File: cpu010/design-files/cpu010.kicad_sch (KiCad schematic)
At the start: 12 parts

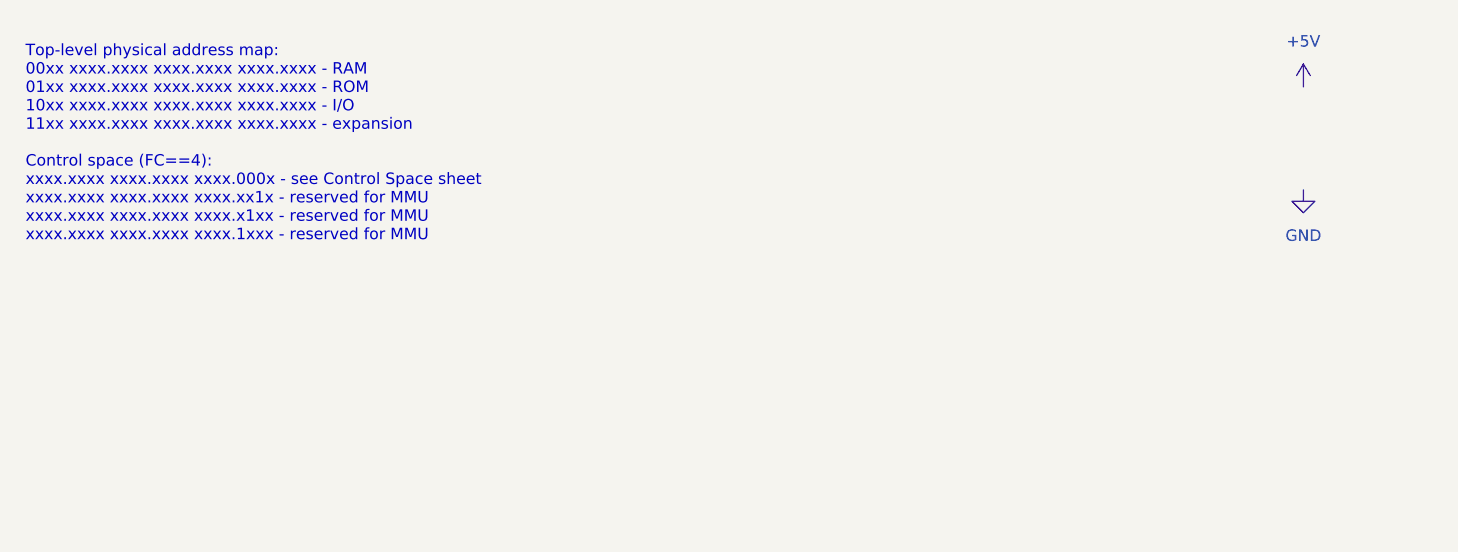
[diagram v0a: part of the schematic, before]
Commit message: More (NQ)VME tweaks.  Add JTAG chain.
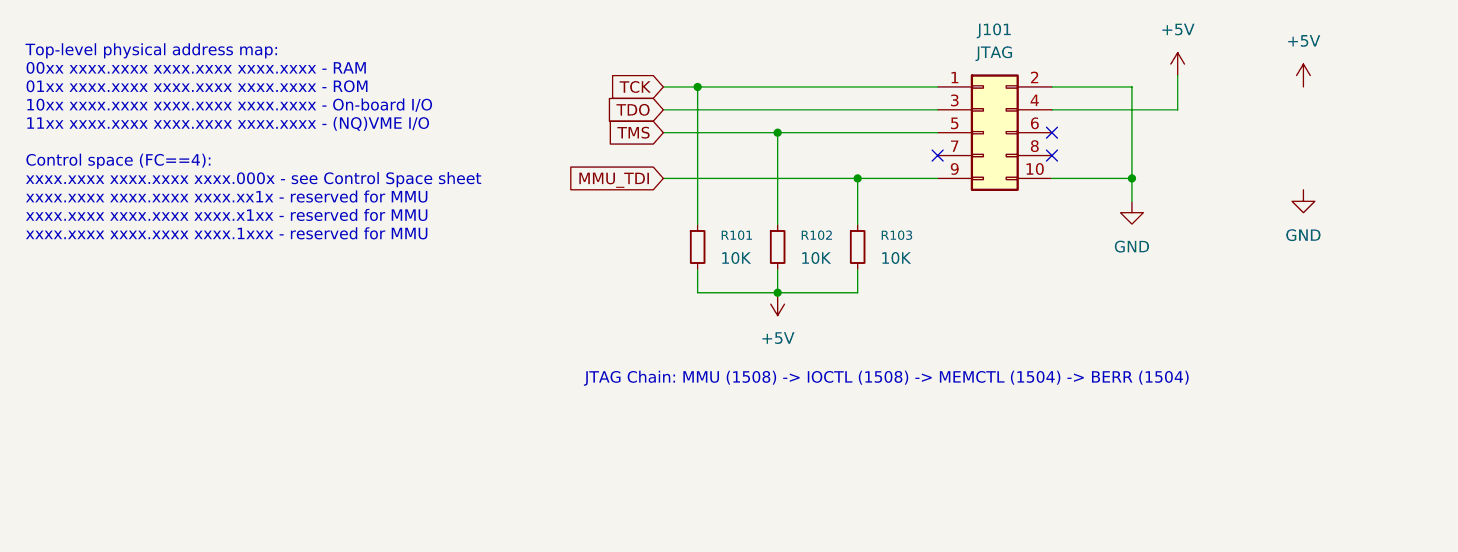
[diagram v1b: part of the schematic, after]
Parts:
- added J101: JTAG, Connector_PinHeader_2.54mm:PinHeader_2x05_P2.54mm_Vertical, symbol Connector_Generic:Conn_02x05_Odd_Even
- added R101, R102, R103: 10K, Resistor_SMD:R_0805_2012Metric_Pad1.20x1.40mm_HandSolder, symbol Device:R_Small
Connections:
- net +5V: now also J101.4 (Pin_4), R101.2, R102.2, R103.2
- net GND: now also J101.10 (Pin_10), J101.2 (Pin_2)
- new net MMU_TDI: J101.9 (Pin_9), R103.1
- new net TCK: J101.1 (Pin_1), R101.1
- new net TDO: J101.3 (Pin_3)
- new net TMS: J101.5 (Pin_5), R102.1
- no-connect marks 0 -> 3
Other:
- note added: "JTAG Chain: MMU (1508) -> IOCTL (1508) -> MEMCTL (1504) -> BERR (1504)"
- note added: "Top-level physical address map: 00xx xxxx.xxxx xxxx.xxxx xxxx.xxxx - RAM 01xx xxxx.xxxx xxxx.xxxx xxxx.xxxx - ROM 10xx xxxx.xxxx xxxx.xxxx xxxx.xxxx - On-board I/O 11xx xxxx.xxxx xxxx.xxxx xxxx.xxxx - (NQ)VME I/O Control space (FC==4): xxxx.xxxx xxxx.xxxx xxxx.000x - see Control Space sheet xxxx.xxxx xxxx.xxxx xxxx.xx1x - reserved for MMU xxxx.xxxx xxxx.xxxx xxxx.x1xx - reserved for MMU xxxx.xxxx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"
- note removed: "Top-level physical address map: 00xx xxxx.xxxx xxxx.xxxx xxxx.xxxx - RAM 01xx xxxx.xxxx xxxx.xxxx xxxx.xxxx - ROM 10xx xxxx.xxxx xxxx.xxxx xxxx.xxxx - I/O 11xx xxxx.xxxx xxxx.xxxx xxxx.xxxx - expansion Control space (FC==4): xxxx.xxxx xxxx.xxxx xxxx.000x - see Control Space sheet xxxx.xxxx xxxx.xxxx xxxx.xx1x - reserved for MMU xxxx.xxxx xxxx.xxxx xxxx.x1xx - reserved for MMU xxxx.xxxx xxxx.xxxx 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"

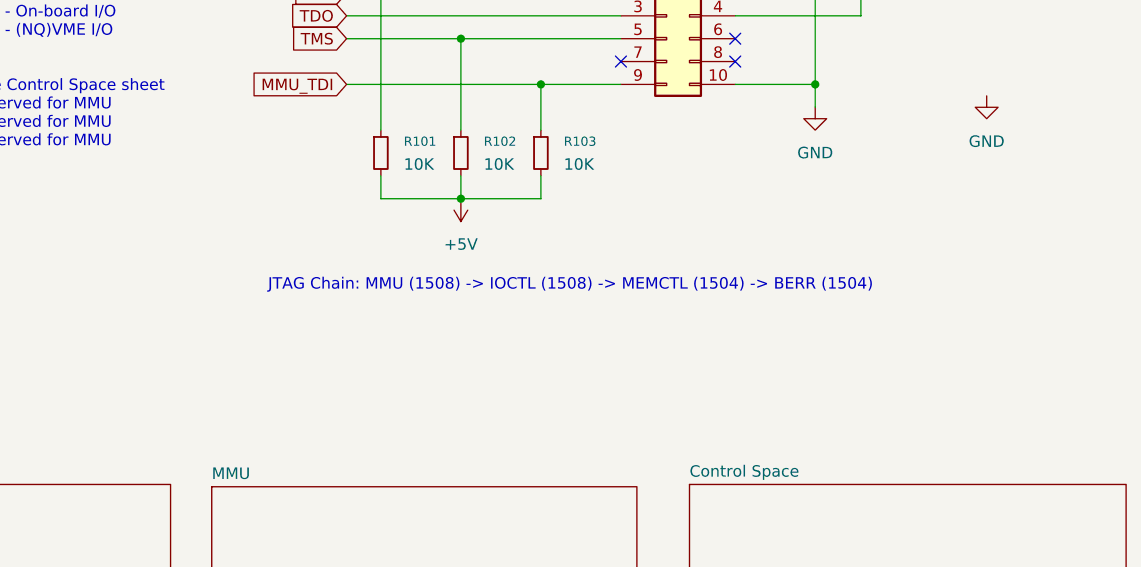
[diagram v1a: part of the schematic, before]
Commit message: Expansion bus changes: - VME bus arb signals are now total no-ops, no daisy-chain. - Ditto for VMS IACK signals. - Neuter some other VME control signals.
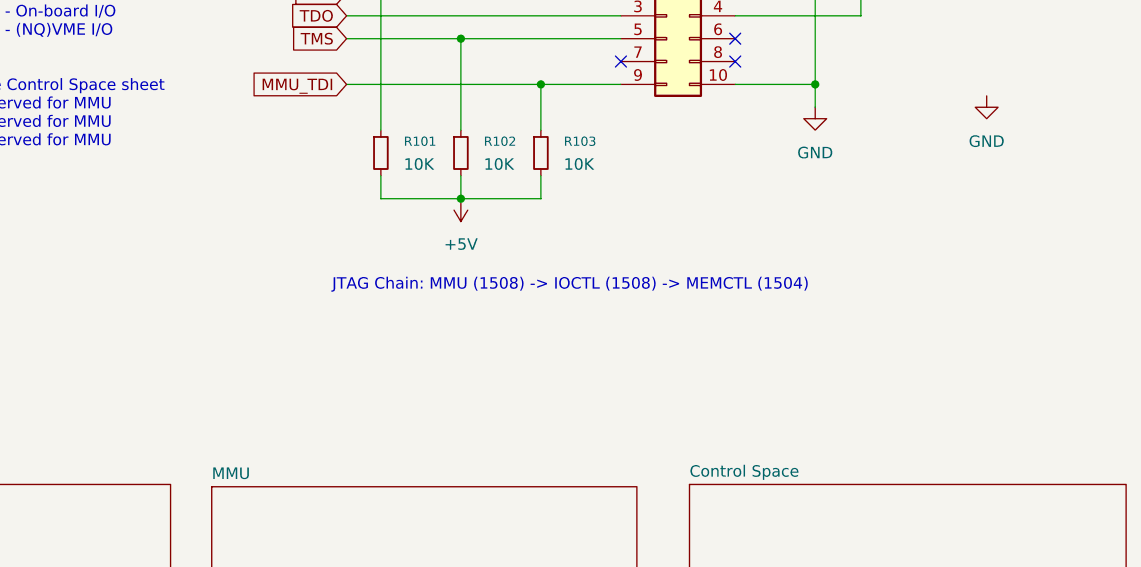
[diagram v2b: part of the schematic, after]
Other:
- note added: "JTAG Chain: MMU (1508) -> IOCTL (1508) -> MEMCTL (1504)"
- note removed: "JTAG Chain: MMU (1508) -> IOCTL (1508) -> MEMCTL (1504) -> BERR (1504)"
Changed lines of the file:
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@@
 		)
 	)
-	(text "JTAG Chain: MMU (1508) -> IOCTL (1508) -> MEMCTL (1504) -> BERR (1504)"
+	(text "JTAG Chain: MMU (1508) -> IOCTL (1508) -> MEMCTL (1504)"
 		(exclude_from_sim no)
 		(at 113.792 55.372 0)
